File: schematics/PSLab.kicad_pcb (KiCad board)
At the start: 4 copper layers, 99 x 53.3 mm, 199 parts, among them J1 DoublePins, J10 Programmer, J11 Battery_Cell, J12 USB_C_Receptacle, J13 CR1225, J2 Conn_01x25, J3 Conn_01x13, J6 ESP01, J8 Micro_SD_Card_Det_9_pin, Q1 MMBT3906, Q2 MMBT3904, Q3 MMBT3906, SW1 SW_MEC_5E, SW2 SW_MEC_5E, SW3 SW_MEC_5E, U1 AP3015A, U10 TL082, U11 TL082, U12 74HC4051, U13 TL082, U14 MCP6S21, U15 CP2102N-xxx-xQFN20x, U16 SP0503BAHT, U17 MT1470, U18 MCP6S21, U2 74HC126, U20 MCP4822, U21 IP5189T, U3 PIC24EP256GP204, U4 DS1307Z+T&R, U6 AMS1117-3.3, U7 LM324, U9 TL082, X1 12MHz, X2 32.768 kHz

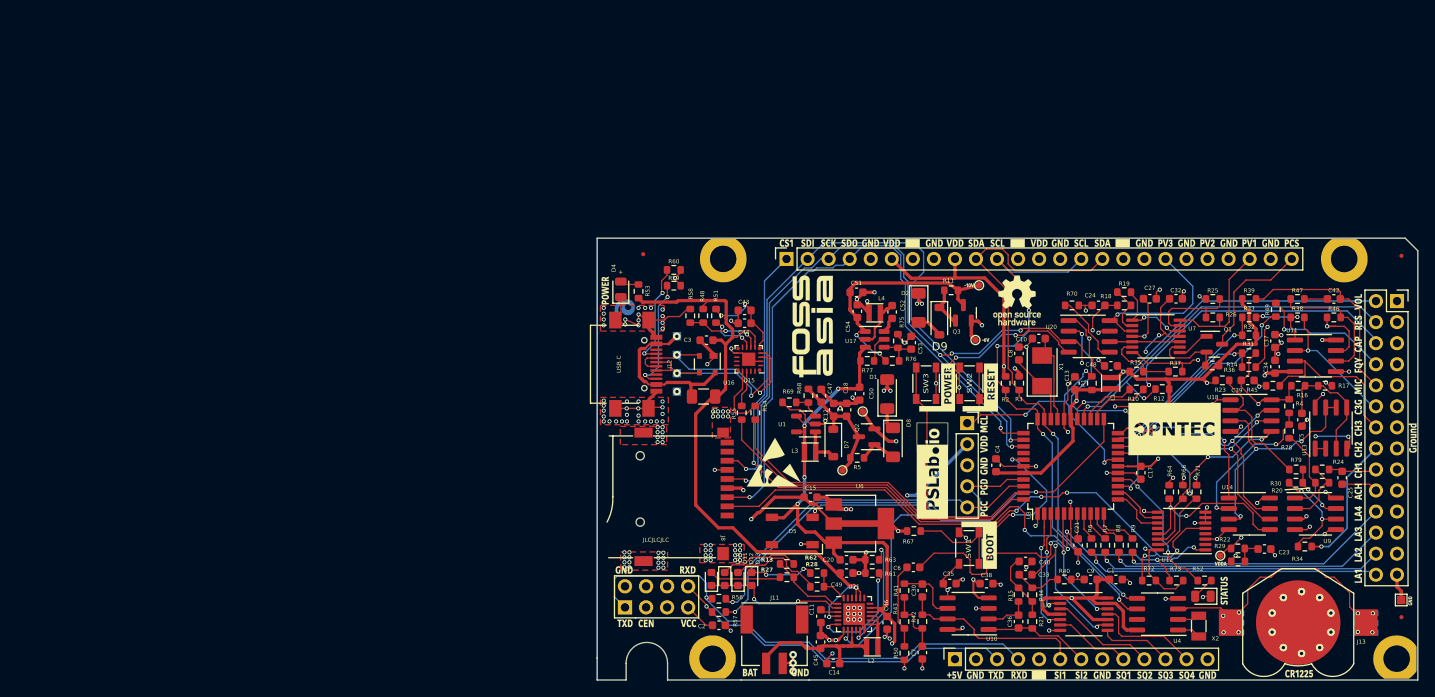
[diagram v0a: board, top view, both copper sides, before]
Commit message: feat: PSLab Mini prototype v1.0
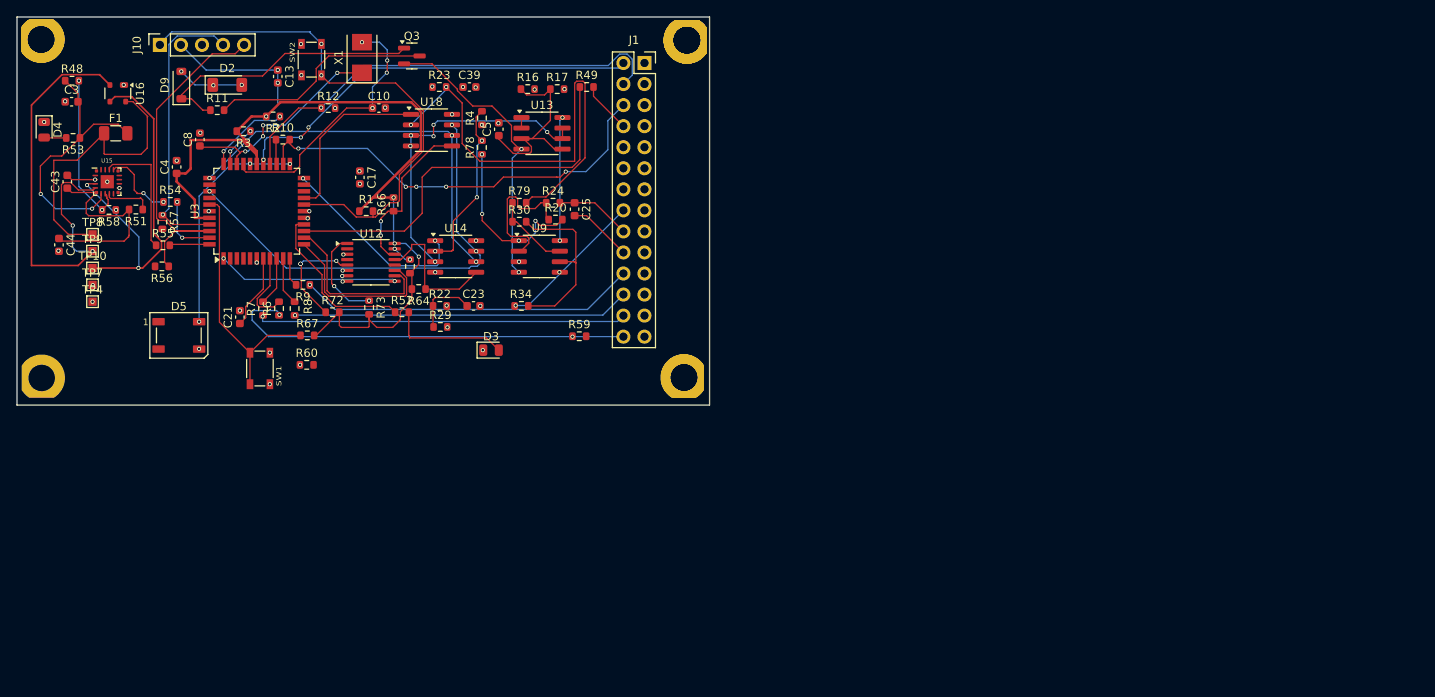
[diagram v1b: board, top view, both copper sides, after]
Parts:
- removed C1, C18, C2, C24, C27, C32, C34, C35, C37, C38, C9: 100nF, Capacitor_SMD:C_0603_1608Metric
- removed C11: 2.2uF, Capacitor_SMD:C_0603_1608Metric
- removed C12, C14, C15, C33, C6: 10uF, Capacitor_SMD:C_0603_1608Metric
- removed C20, C42, C52: 1uF, Capacitor_SMD:C_0603_1608Metric
- removed C30, C36: 1nF, Capacitor_SMD:C_0603_1608Metric
- removed C40, C7: 10nF, Capacitor_SMD:C_0603_1608Metric
- removed C45, C46, C47, C48, C49, C50, C51, C54: 22uF, Capacitor_SMD:C_0603_1608Metric
- removed C53: 12pF, Capacitor_SMD:C_0603_1608Metric
- removed D1: 6.8V, Diode_SMD:D_MiniMELF
- removed D10, D11, D12, D13: White, LED_SMD:LED_0603_1608Metric
- removed D7: K1N5817HW-7-F, Diode_SMD:D_SOD-123
- removed D8: 1N4148W, Diode_SMD:D_MiniMELF
- removed FID1, FID2, FID3: Fiducial, Fiducial:Fiducial_0.5mm_Mask1.5mm
- removed J11: Battery_Cell, PSLab:2.0mm_connector_edge
- removed J12: USB_C_Receptacle, PSLab:USB_C_Receptacle_12pin_SMT
- removed J13: CR1225, PSLab:BatteryHolder_A359
- removed J2: Conn_01x25, Connector_PinSocket_2.54mm:PinSocket_1x25_P2.54mm_Vertical
- removed J3: Conn_01x13, Connector_PinSocket_2.54mm:PinSocket_1x13_P2.54mm_Vertical
- removed J6: ESP01, PSLab:ESP-01
- removed J8: Micro_SD_Card_Det_9_pin, PSLab:TF-015
- removed L1, L3, L4: 3.3uH, Inductor_SMD:L_Taiyo-Yuden_MD-2020
- removed L2: 4.7uH, Inductor_SMD:L_Taiyo-Yuden_MD-2020
- removed MH1, MH2, MH3: M, PSLab:OneSided_MPad
- removed the MH4 at (196.5, 97.4)
- removed Q1: MMBT3906, Package_TO_SOT_SMD:SOT-23
- removed Q2: MMBT3904, Package_TO_SOT_SMD:SOT-23
- removed R13, R27, R28, R62: 200, Resistor_SMD:R_0603_1608Metric
- removed R14, R18, R19, R21, R25, R31, R32, R33, R35, R37, R38, R39, R42, R70, R76: 10k, Resistor_SMD:R_0603_1608Metric
- removed R15, R26, R41, R43, R44: 5.1k, Resistor_SMD:R_0603_1608Metric
- removed R36, R47, R5: 1k, Resistor_SMD:R_0603_1608Metric
- removed R40, R46, R50, R63, R77: 200k, Resistor_SMD:R_0603_1608Metric
- removed R45: 1M, Resistor_SMD:R_0603_1608Metric
- removed R61: 51k, Resistor_SMD:R_0603_1608Metric
- removed R68: 180k, Resistor_SMD:R_0603_1608Metric
- removed R69: 30k, Resistor_SMD:R_0603_1608Metric
- removed R75: 100k, Resistor_SMD:R_0603_1608Metric
- removed SW3: SW_MEC_5E, PSLab:button_SPST_3x4x2.5
- removed TP1, TP2, TP3, TP5, TP6: TEST, PSLab:Test_Point_0.8mm
- removed U1: AP3015A, Package_TO_SOT_SMD:SOT-23-5
- removed U10, U11: TL082, Package_SO:SOIC-8_3.9x4.9mm_P1.27mm
- removed U17: MT1470, Package_TO_SOT_SMD:SOT-23-6
- removed U2: 74HC126, Package_SO:TSSOP-14_4.4x5mm_P0.65mm
- removed U20: MCP4822, Package_SO:SOIC-8_3.9x4.9mm_P1.27mm
- removed U21: IP5189T, Package_DFN_QFN:QFN-24-1EP_4x4mm_P0.5mm_EP2.6x2.6mm
- removed U4: DS1307Z+T&R, Package_SO:SOIC-8_3.9x4.9mm_P1.27mm
- removed U6: AMS1117-3.3, Package_TO_SOT_SMD:SOT-223-3_TabPin2
- removed U7: LM324, Package_SO:TSSOP-14_4.4x5mm_P0.65mm
- removed X2: 32.768 kHz, Crystal:Crystal_SMD_3215-2Pin_3.2x1.5mm
- removed Z1: CR1225, Battery:Battery_CR1225
- removed Z10: ESD-Logo, Symbol:ESD-Logo_6.6x6mm_SilkScreen
- removed Z11 (x2): OpenHardware, Symbol:OSHW-Logo_5.7x6mm_SilkScreen
- removed Z6: eWaste, Symbol:WEEE-Logo_4.2x6mm_SilkScreen
- removed Z7: PSLab BarCode, PSLab:Barcode
- removed Z9: Silk, PSLab:PSLab_SilkScreen
- added ?: , , F.Cu at (110.5, 63.5)
- added ? (x3): , , F.Cu at (110.8, 22.8)
- added ?: , , F.Cu at (32.9, 22.7)
- added MH4: M, PSLab:TwoSided_MPad, F.Cu at (33.0, 63.6)
- added MH4: M, PSLab:TwoSided_MPad, F.Cu at (110.8, 22.8)
- added MH4: M, PSLab:TwoSided_MPad, F.Cu at (32.9, 22.7)
- added MH4: M, PSLab:TwoSided_MPad, F.Cu at (110.5, 63.5)
- D5: footprint PSLab:LED_WS2812B_PLCC4_5.0x5.0mm_P3.2mm -> LED_SMD:LED_WS2812B_PLCC4_5.0x5.0mm_P3.2mm
- TP10, TP7, TP8, TP9: moved to F.Cu
- moved TP4 162.0 mm to (39.1, 54.4)
- moved J10 107.6 mm to (47.2, 23.4), turned to 90 degrees
- moved R10 107.3 mm to (62.1, 34.8)
- moved R12 106.2 mm to (67.6, 31.0)
- moved R7 105.6 mm to (59.7, 55.2)
- moved C4 105.2 mm to (49.3, 38.1)
- moved R9 104.9 mm to (64.5, 52.3), turned to 180 degrees
- moved C21 104.8 mm to (56.9, 56.2), turned to 90 degrees
- moved U18 104.7 mm to (80.0, 33.7)
- moved R72 103.7 mm to (68.1, 55.6)
- moved R8 103.5 mm to (63.5, 55.2)
- moved R4 103.4 mm to (86.1, 32.2), turned to 90 degrees
- moved R78 103.2 mm to (86.1, 35.8)
- moved C13 103.1 mm to (61.5, 27.2), turned to -90 degrees
- moved U12 103.1 mm to (72.7, 49.6), turned to 0 degrees
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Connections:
- net SCL renamed /SCL
- net SD.CS renamed Net-(U12-A5)
- net SDA renamed /SDA
- J1 pad 10: MIC -> unconnected-(J1-Pin_10-Pad10)
- J1 pad 12: CH3.GAIN -> unconnected-(J1-Pin_12-Pad12)
- J1 pad 14: CH3 -> unconnected-(J1-Pin_14-Pad14)
- U3 pad 20: CH3_IN -> unconnected-(U3-AN1|C2IN1+|RA1-Pad20)
- U3 pad 21: MIC_IN -> unconnected-(U3-PGED3|AN2|C2IN1-|RPI32|RB0-Pad21)
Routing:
- net GND: track 178.1 -> 3.57 mm, vias 178 -> 56
- net +6V: track 136.5 -> 15.0 mm, vias 8 -> 2
- net +5V: track 118.3 -> 0.00 mm, vias 6 -> 0
- net VDDA: track 108.4 -> 0.00 mm, vias 9 -> 10
- net -6V: track 131.1 -> 35.3 mm, vias 8 -> 2
- net SDO: track 141.0 -> 48.2 mm, vias 9 -> 3
- net SPI.CS: track 95.2 -> 11.5 mm, vias 6 -> 2
- net SCK: track 138.0 -> 54.9 mm, vias 10 -> 3
- net SDI: track 76.9 -> 0.00 mm, vias 2 -> 0
- net +3.3V: track 201.2 -> 125.6 mm, vias 11 -> 5
- net /SDA: track 68.6 -> 4.96 mm
- net RxD2: track 60.3 -> 0.00 mm, vias 1 -> 0
- net Net-(U12-A5): track 72.4 -> 13.1 mm, vias 5 -> 3
- net /SCL: track 67.0 -> 10.1 mm, vias 4 -> 2
- net /VINPUT: track 78.8 -> 33.2 mm
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- removed copper zone on F.Cu, net GND
- removed copper zone on B.Cu, net Net-(J13-+)
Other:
- board size 99 x 53.3 mm -> 83.6 x 46.8 mm
- board text added: "{ "ViaStitching": "0.2", "stitch_zone_0": { "HSpacing": "1", "VSpacing": "1", "HOffset": "0", "VOffset": "0", "Clearance": "0", "Randomize": false } }"
- board text removed: "+"
- board text removed: "JLCJLCJLC"
- board text removed: "USB C"
